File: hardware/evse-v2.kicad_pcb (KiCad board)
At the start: 4 copper layers, 74 x 114 mm, 143 parts, among them J101 Boot, P101 CON-SENSOR2, P102 Relay, P103 L'+PE, P104 L'+PE, P105 CP/PP/PE, P106 Power, P107 Motor, P108 Switch_LED, P109 Enable, P110 MODBUS, P111 Debug, P112 DC-Protect, P113 GP, Q101 2N7002P, Q102 SI2305CDS-T1-GE3, Q103 2N7002P, Q104 2N7002P, Q105 SSM3J355R,LF, SW101 OS103011MS8QP1, SW102 OS103011MS8QP1, U101 XMC1404, U102 PEM1-S12-D12-S, U103 DMMT5401, U105 OPA171AIDBV, U106 A5950GLP, U108 AQH3213AX, U109 HCPL2731, U110 TPS70933DBVR, U111 IRM02-12, U112 WPMDL110, U113 SP3491, X101 16MHz

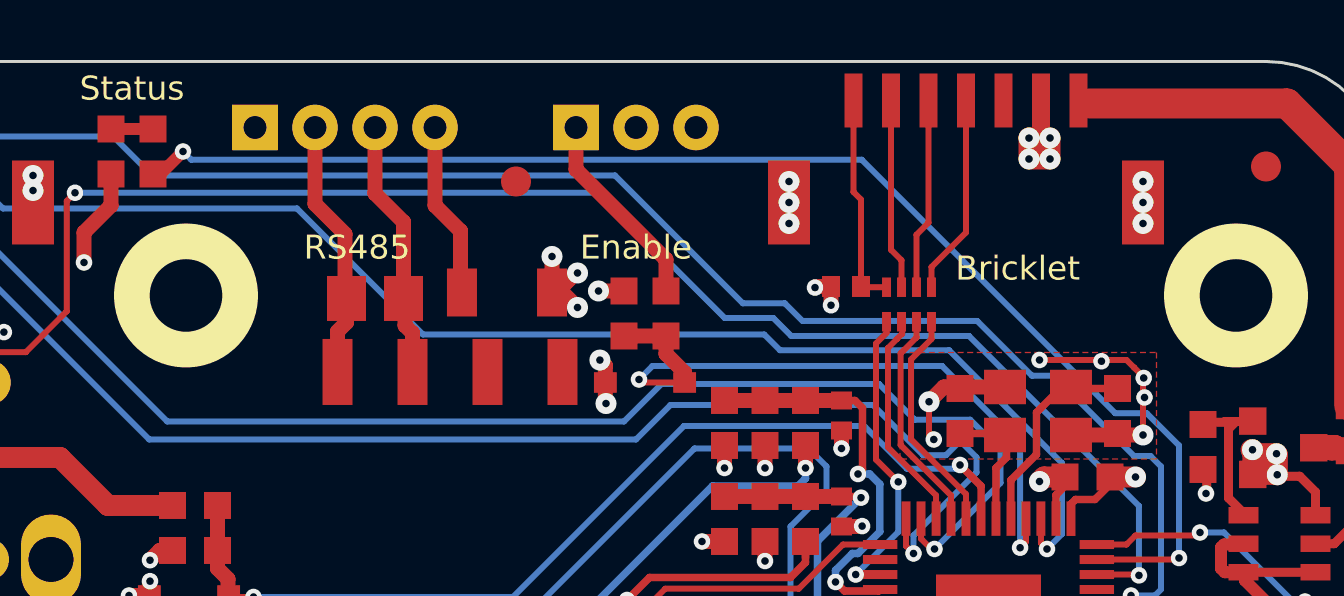
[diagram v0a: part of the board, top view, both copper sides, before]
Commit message: ordered prototype
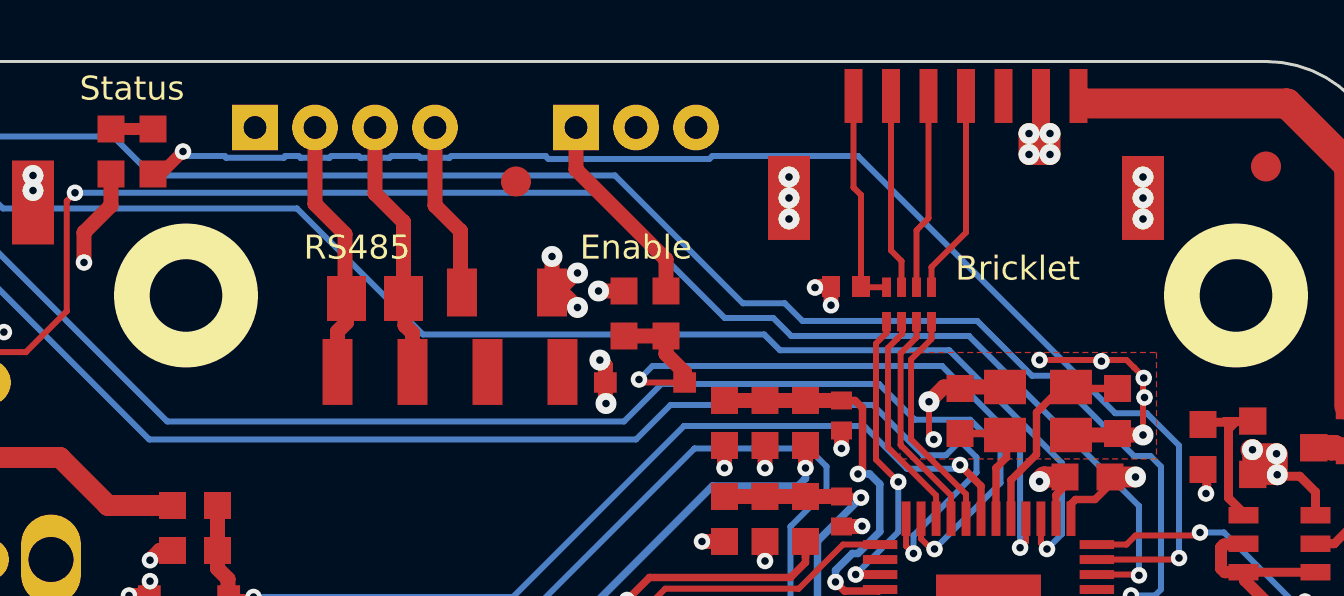
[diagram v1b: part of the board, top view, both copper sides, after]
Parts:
- moved P101 0.15 mm to (137.3, 57.5)
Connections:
- RP105 pad 2: AC1 -> AC2
- RP105 pad 3: AC2 -> AC1
- U101 pad 10: AC1 -> AC2
- U101 pad 9: AC2 -> AC1
